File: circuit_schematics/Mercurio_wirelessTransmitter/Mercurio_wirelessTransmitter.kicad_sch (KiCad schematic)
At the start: 1 part

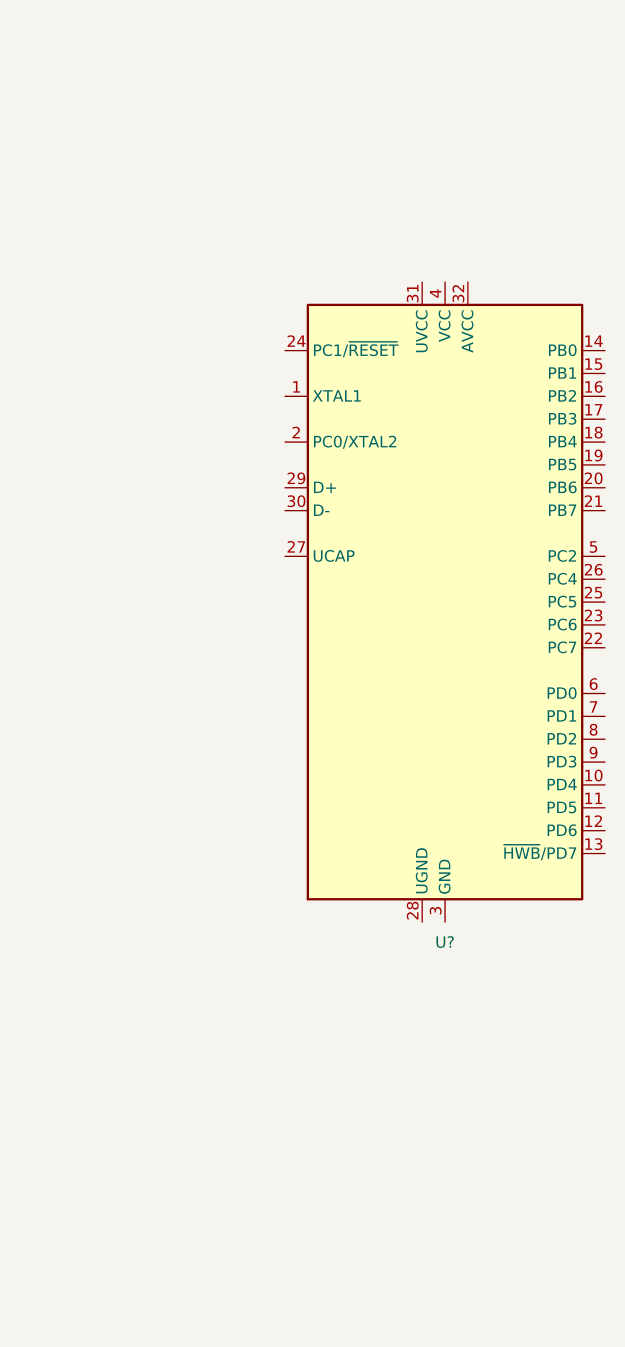
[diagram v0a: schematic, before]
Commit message: Alteracoes ao esquematico.
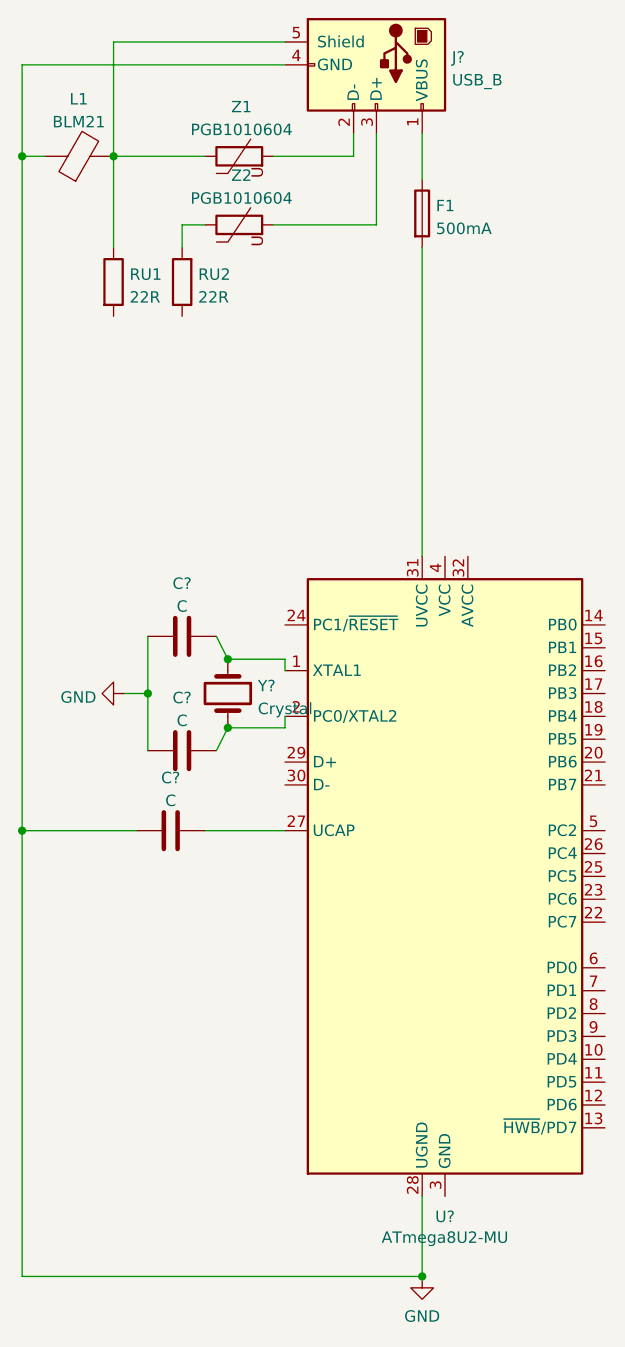
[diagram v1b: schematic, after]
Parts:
- added C? (x3): C, symbol Device:C
- added F1: 500mA, symbol Device:Fuse
- added J?: USB_B, symbol Connector:USB_B
- added L1: BLM21, symbol Device:FerriteBead
- added RU1, RU2: 22R, symbol Device:R
- added Y?: Crystal, symbol Device:Crystal
- added Z1, Z2: PGB1010604, symbol Device:Varistor
- U?: value (none) -> ATmega8U2-MU; footprint (none) -> Package_DFN_QFN:QFN-32-1EP_5x5mm_P0.5mm_EP3.1x3.1mm
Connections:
- net at U?.1 (XTAL1): now also C?.2, Y?.1
- net at U?.2 (PC0/XTAL2): now also C?.2, Y?.2
- net at U?.27 (UCAP): now also C?.2
- net GND: now reaches U?.28 (UGND)
- net GND: now also C?.1, C?.1, C?.1, J?.4 (GND), L1.1
- net at U?.31 (UVCC): now also F1.2
- new net: RU2.2, Z2.1
- new net: F1.1, J?.1 (VBUS)
- new net: J?.5 (Shield), L1.2, RU1.1, Z1.1
- new net: J?.2 (D-), Z1.2
- new net: J?.3 (D+), Z2.2
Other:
- moved on the sheet: U?
